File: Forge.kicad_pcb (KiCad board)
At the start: 2 copper layers, 10 parts, among them J1 USB_C_Receptacle_USB2.0_14P, U1 ESP32-S3-WROOM-2, U2 AP2112K-3.3, U3 USBLC6-2SC6

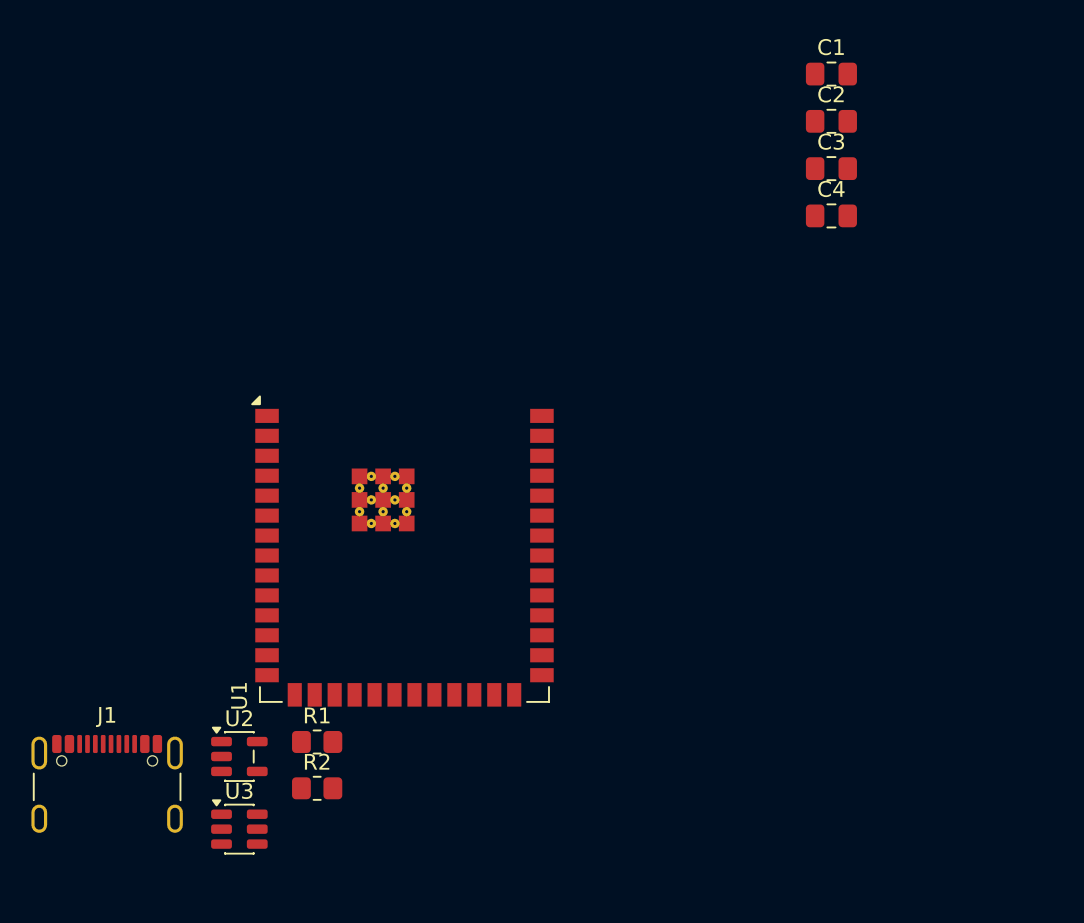
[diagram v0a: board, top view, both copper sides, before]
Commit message: Finished schematic ready for review
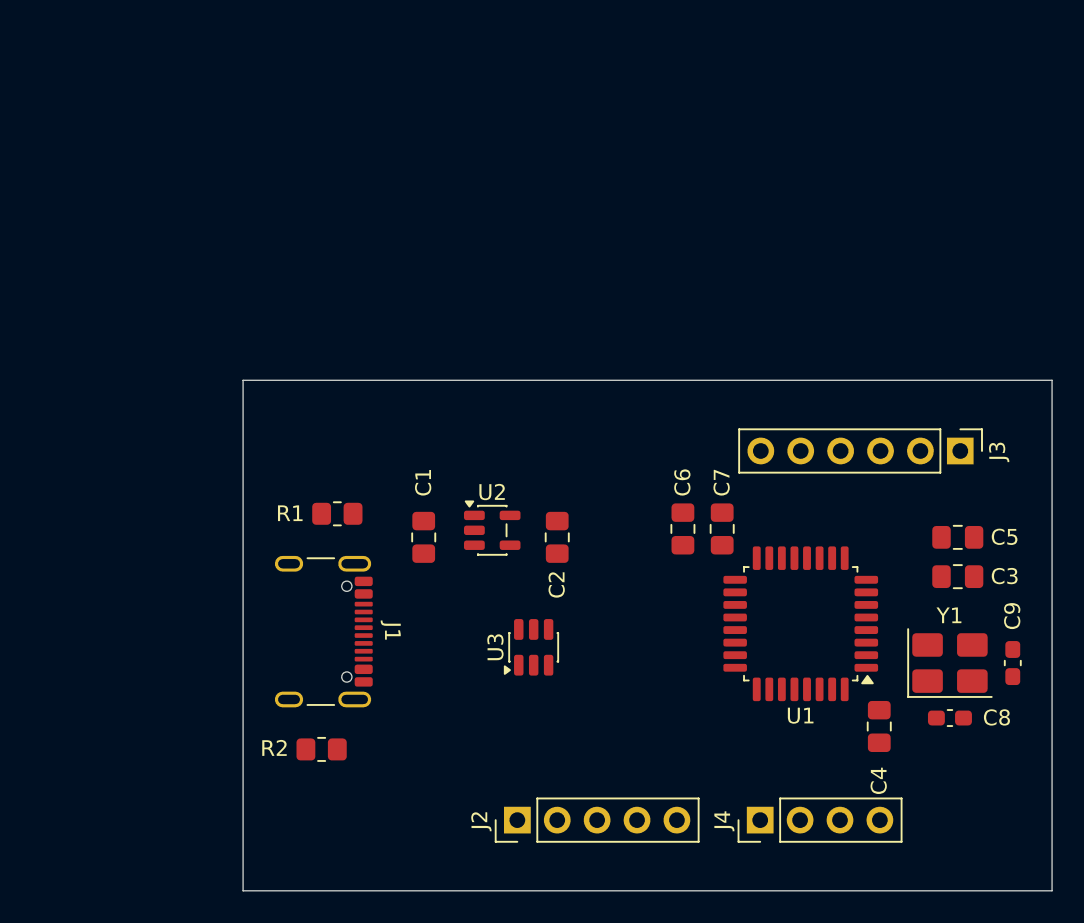
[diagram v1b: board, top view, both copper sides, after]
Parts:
- added C5: 100n, Capacitor_SMD:C_0805_2012Metric_Pad1.18x1.45mm_HandSolder, F.Cu at (161.5, 69.0)
- added C6: 100n, Capacitor_SMD:C_0805_2012Metric_Pad1.18x1.45mm_HandSolder, F.Cu at (144.0, 68.5)
- added C7: 10u, Capacitor_SMD:C_0805_2012Metric_Pad1.18x1.45mm_HandSolder, F.Cu at (146.5, 68.5)
- added C8: 100n, Capacitor_SMD:C_0603_1608Metric_Pad1.08x0.95mm_HandSolder, F.Cu at (161.0, 80.5)
- added C9: 100n, Capacitor_SMD:C_0603_1608Metric_Pad1.08x0.95mm_HandSolder, F.Cu at (165.0, 77.0)
- added J2: SWD, Connector_PinHeader_2.54mm:PinHeader_1x05_P2.54mm_Vertical, F.Cu at (133.5, 87.0)
- added J3: SPI, Connector_PinHeader_2.54mm:PinHeader_1x06_P2.54mm_Vertical, F.Cu at (161.7, 63.5)
- added J4: I2C, Connector_PinHeader_2.54mm:PinHeader_1x04_P2.54mm_Vertical, F.Cu at (148.9, 87.0)
- added Y1: Crystal_GND24, Crystal:Crystal_SMD_EuroQuartz_MT-4Pin_3.2x2.5mm_HandSoldering, F.Cu at (161.0, 77.0)
- C4: value 10u -> 100n
- U1: value ESP32-S3-WROOM-2 -> STM32F042K6Tx; footprint RF_Module:ESP32-S3-WROOM-2 -> Package_QFP:LQFP-32_7x7mm_P0.8mm
- moved C1 39.3 mm to (127.5, 69.0), turned to 90 degrees
- moved C4 32.6 mm to (156.5, 81.0), turned to -90 degrees
- moved C2 31.7 mm to (136.0, 69.0), turned to -90 degrees
- moved C3 27.2 mm to (161.5, 71.5)
- moved U1 26.5 mm to (151.5, 74.5), turned to 180 degrees
- moved U3 22.0 mm to (134.5, 76.0), turned to 90 degrees
- moved U2 21.6 mm to (131.9, 68.5)
- moved J1 16.7 mm to (120.0, 75.0), turned to -90 degrees
- moved R1 14.6 mm to (122.0, 67.5), turned to 180 degrees
- moved R2 2.49 mm to (121.0, 82.5), turned to 180 degrees
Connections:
- C3 pad 1: +3.3V -> NRST
- U1 pad 1: GND -> +3.3V
- U1 pad 10: unconnected-(U1-IO17-Pad10) -> SPI_NSS
- U1 pad 11: unconnected-(U1-IO18-Pad11) -> SPI_SCK
- U1 pad 12: I2C_SDA -> SPI_MISO
- U1 pad 13: USB_D- -> SPI_MOSI
- U1 pad 14: USB_D+ -> unconnected-(U1-PB0-Pad14)
- U1 pad 16: unconnected-(U1-IO46-Pad16) -> GND
- U1 pad 17: I2C_SCL -> +3.3V
- U1 pad 18: SPI_CLK -> unconnected-(U1-PA8-Pad18)
- U1 pad 19: SPI_MOSI -> unconnected-(U1-PA9-Pad19)
- U1 pad 2: +3.3V -> OSC_IN
- U1 pad 20: SPI_MISO -> unconnected-(U1-PA10-Pad20)
- U1 pad 21: SPI_CS -> USB_D-
- U1 pad 22: unconnected-(U1-IO14-Pad22) -> USB_D+
- U1 pad 23: unconnected-(U1-IO21-Pad23) -> SWDIO
- U1 pad 24: unconnected-(U1-IO47-Pad24) -> SWCLK
- U1 pad 29: unconnected-(U1-NC-Pad29) -> I2C_SCL
- U1 pad 3: unconnected-(U1-EN-Pad3) -> OSC_OUT
- U1 pad 30: unconnected-(U1-NC-Pad30) -> I2C_SDA
- U1 pad 31: unconnected-(U1-IO38-Pad31) -> BOOT0
- U1 pad 32: unconnected-(U1-MTCK/IO39-Pad32) -> GND
- U1 pad 4: unconnected-(U1-IO4-Pad4) -> NRST
- U1 pad 5: unconnected-(U1-IO5-Pad5) -> +3.3V
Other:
- board outline added: 51.5 x 32.5 mm
